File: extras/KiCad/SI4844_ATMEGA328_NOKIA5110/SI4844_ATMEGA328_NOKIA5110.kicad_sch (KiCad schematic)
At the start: 18 parts, among them J1 AudioJack2_Ground, U1 Nokia_5110_LCD, Y1 Crystal

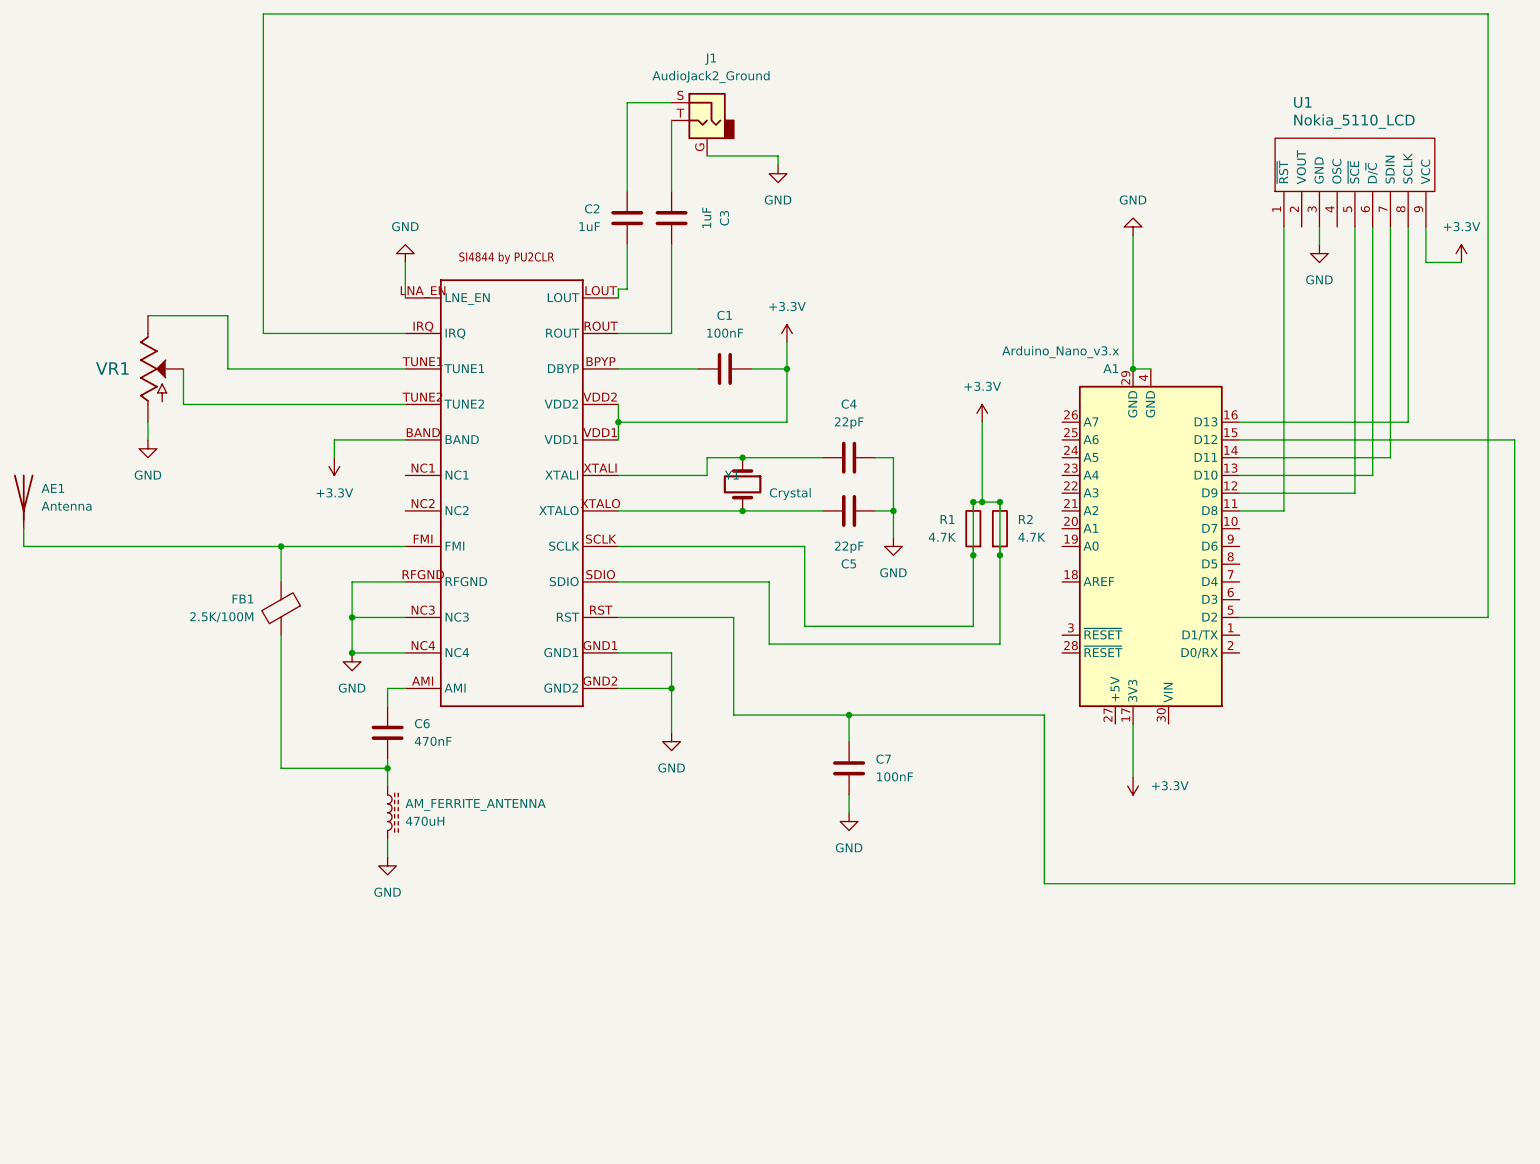
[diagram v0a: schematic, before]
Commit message: Doc
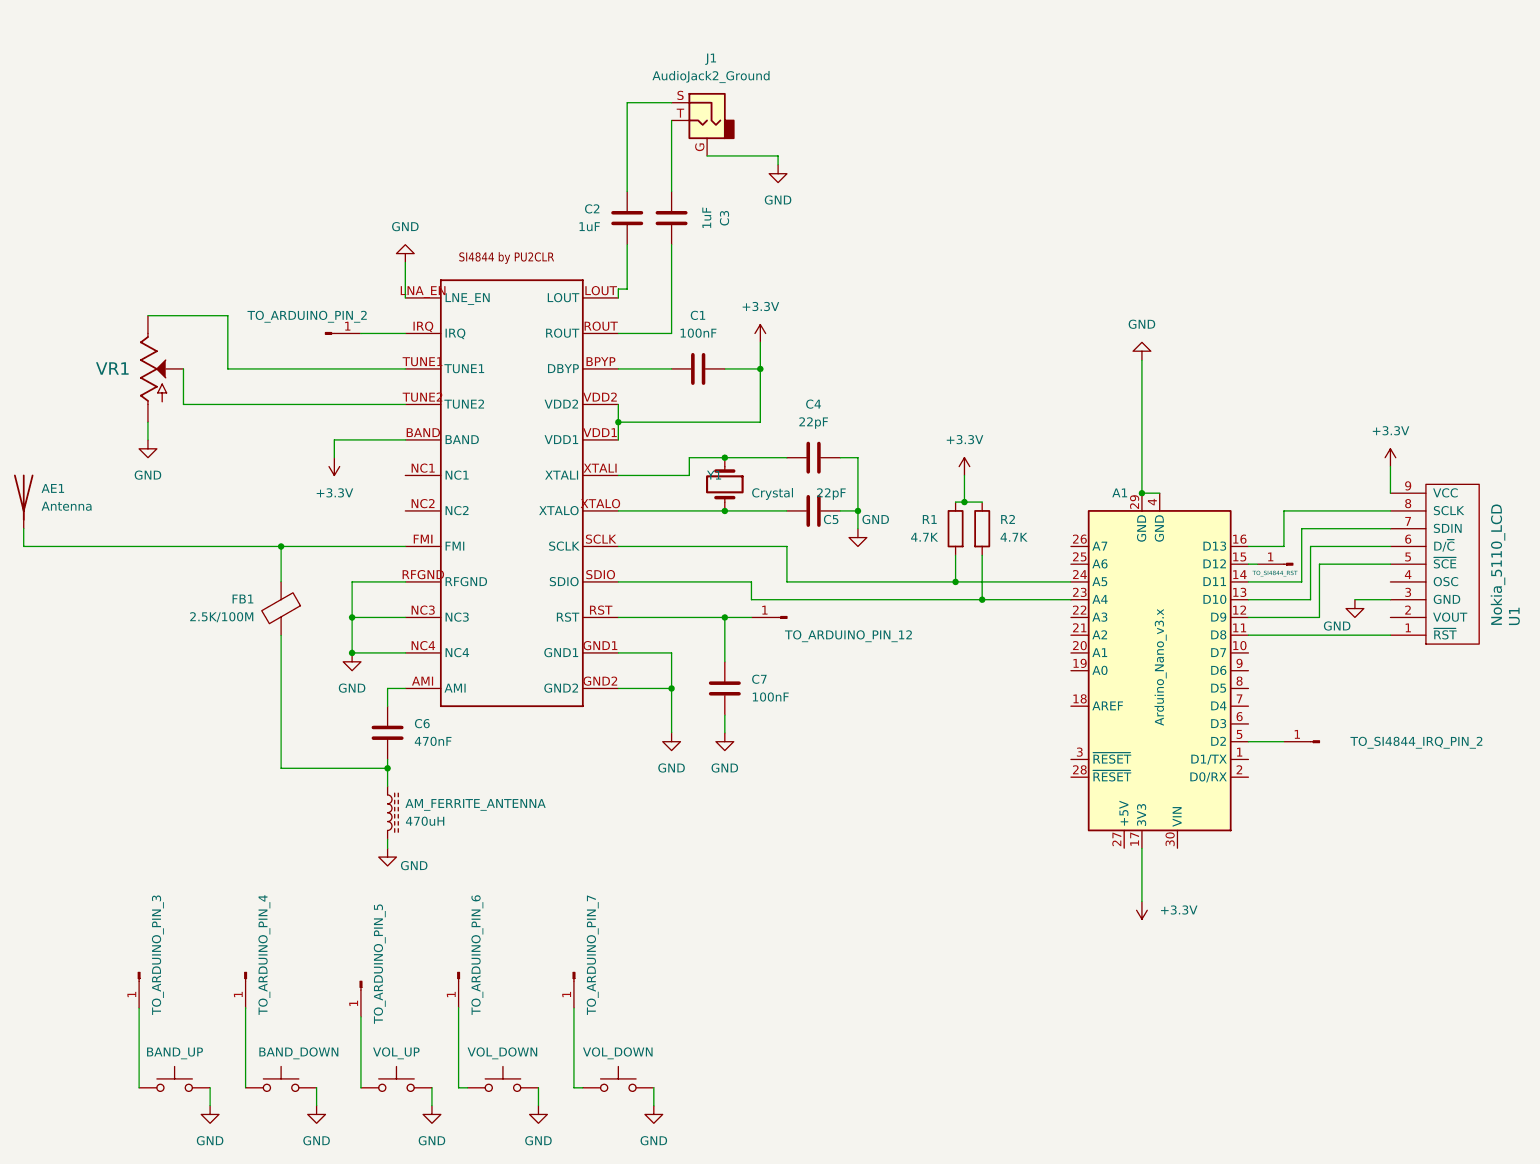
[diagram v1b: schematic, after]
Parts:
- added J10: TO_ARDUINO_PIN_7, symbol Connector:Conn_01x01_Pin
- added J2: TO_SI4844_IRQ_PIN_2, symbol Connector:Conn_01x01_Pin
- added J3: TO_ARDUINO_PIN_2, symbol Connector:Conn_01x01_Pin
- added J4: TO_ARDUINO_PIN_12, symbol Connector:Conn_01x01_Pin
- added J5: TO_SI4844_RST, symbol Connector:Conn_01x01_Pin
- added J6: TO_ARDUINO_PIN_3, symbol Connector:Conn_01x01_Pin
- added J7: TO_ARDUINO_PIN_4, symbol Connector:Conn_01x01_Pin
- added J8: TO_ARDUINO_PIN_5, symbol Connector:Conn_01x01_Pin
- added J9: TO_ARDUINO_PIN_6, symbol Connector:Conn_01x01_Pin
- added SW1: BAND_UP, symbol Switch:SW_Push
- added SW2: BAND_DOWN, symbol Switch:SW_Push
- added SW3: VOL_UP, symbol Switch:SW_Push
- added SW4, SW5: VOL_DOWN, symbol Switch:SW_Push
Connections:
- net +3.3V: no longer R1.2, R2.2, SI1.SCLK, SI1.SDIO
- net GND: now also SW1.2, SW2.2, SW3.2, SW4.2, SW5.2
- net at C7.1, SI1.RST: now also J4.1 (Pin_1); no longer A1.15 (D12)
- net at A1.23 (A4): now also R2.2, SI1.SDIO
- net at A1.24 (A5): now also R1.2, SI1.SCLK
- net at A1.5 (D2): now also J2.1 (Pin_1); no longer SI1.IRQ
- new net: J10.1 (Pin_1), SW5.1
- new net: A1.15 (D12), J5.1 (Pin_1)
- new net: J3.1 (Pin_1), SI1.IRQ
- new net: J6.1 (Pin_1), SW1.1
- new net: J9.1 (Pin_1), SW4.1
- new net: J7.1 (Pin_1), SW2.1
- new net: J8.1 (Pin_1), SW3.1
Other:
- title: SI4844 and Arduino Setup -> SI4844, NOKIA 5110  and Arduino Setup
- moved on the sheet: A1, C1, C4, C5, C7, R1, R2, U1, Y1
